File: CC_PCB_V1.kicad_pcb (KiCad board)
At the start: 2 copper layers, 7 parts, among them J1 Screw_Terminal_01x02, J2 Antenna_Conn_02x04_Odd_Even, J3 USB1130-15-A_REVA, J5 Relay_Conn_01x06, U1 Pico, U2 level_converter_BOB-12009

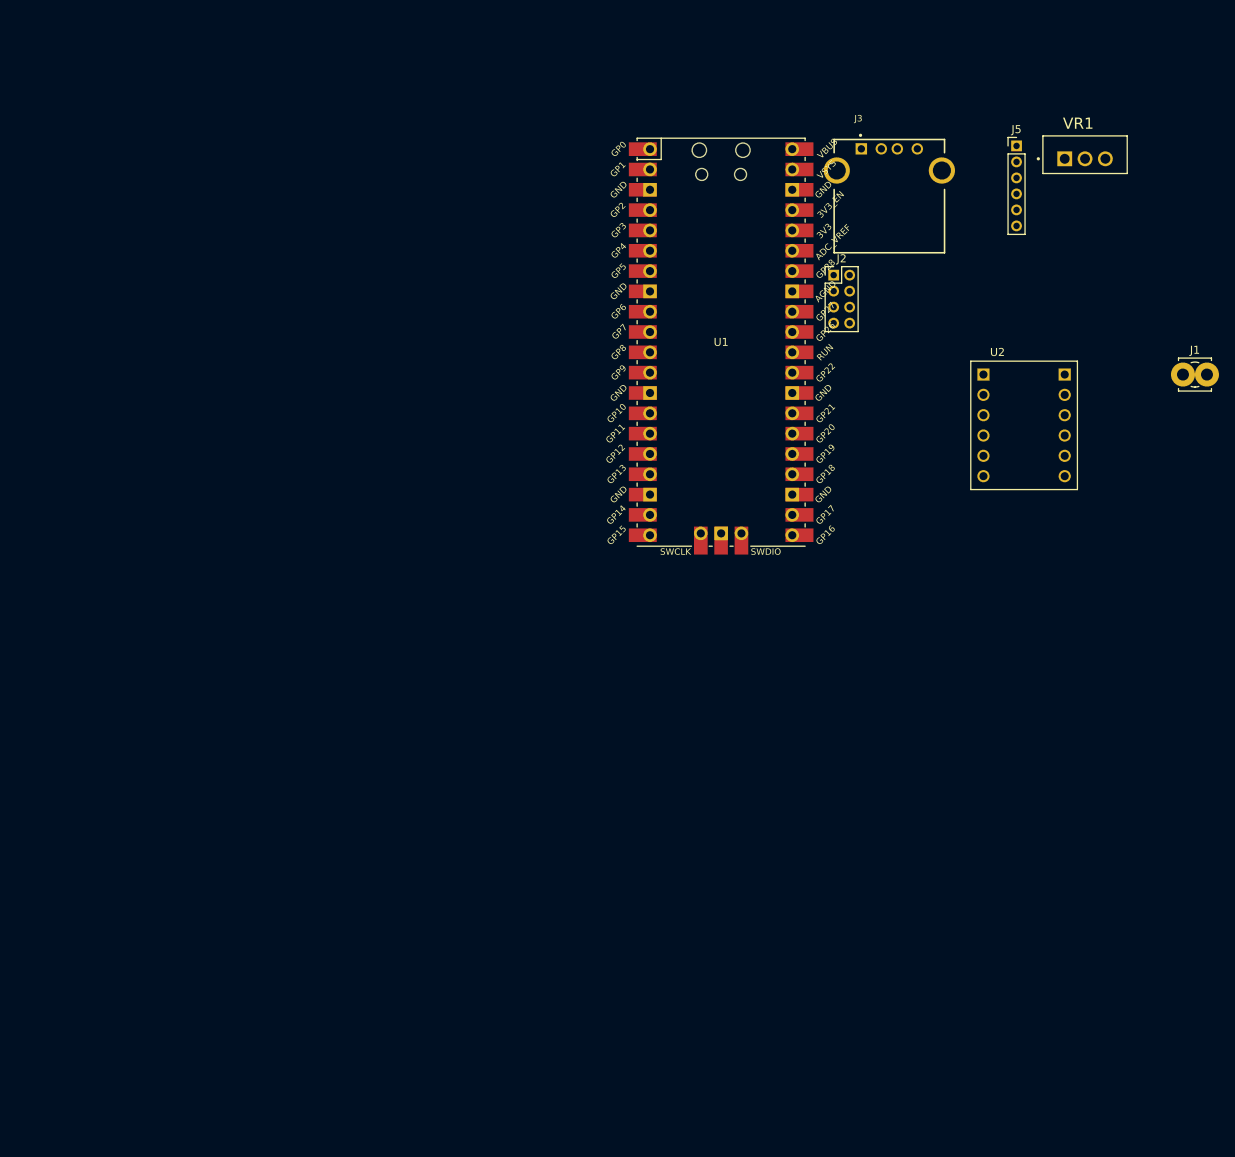
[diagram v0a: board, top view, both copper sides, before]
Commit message: Wiring Board
I tried my best here,  let me know what you think.
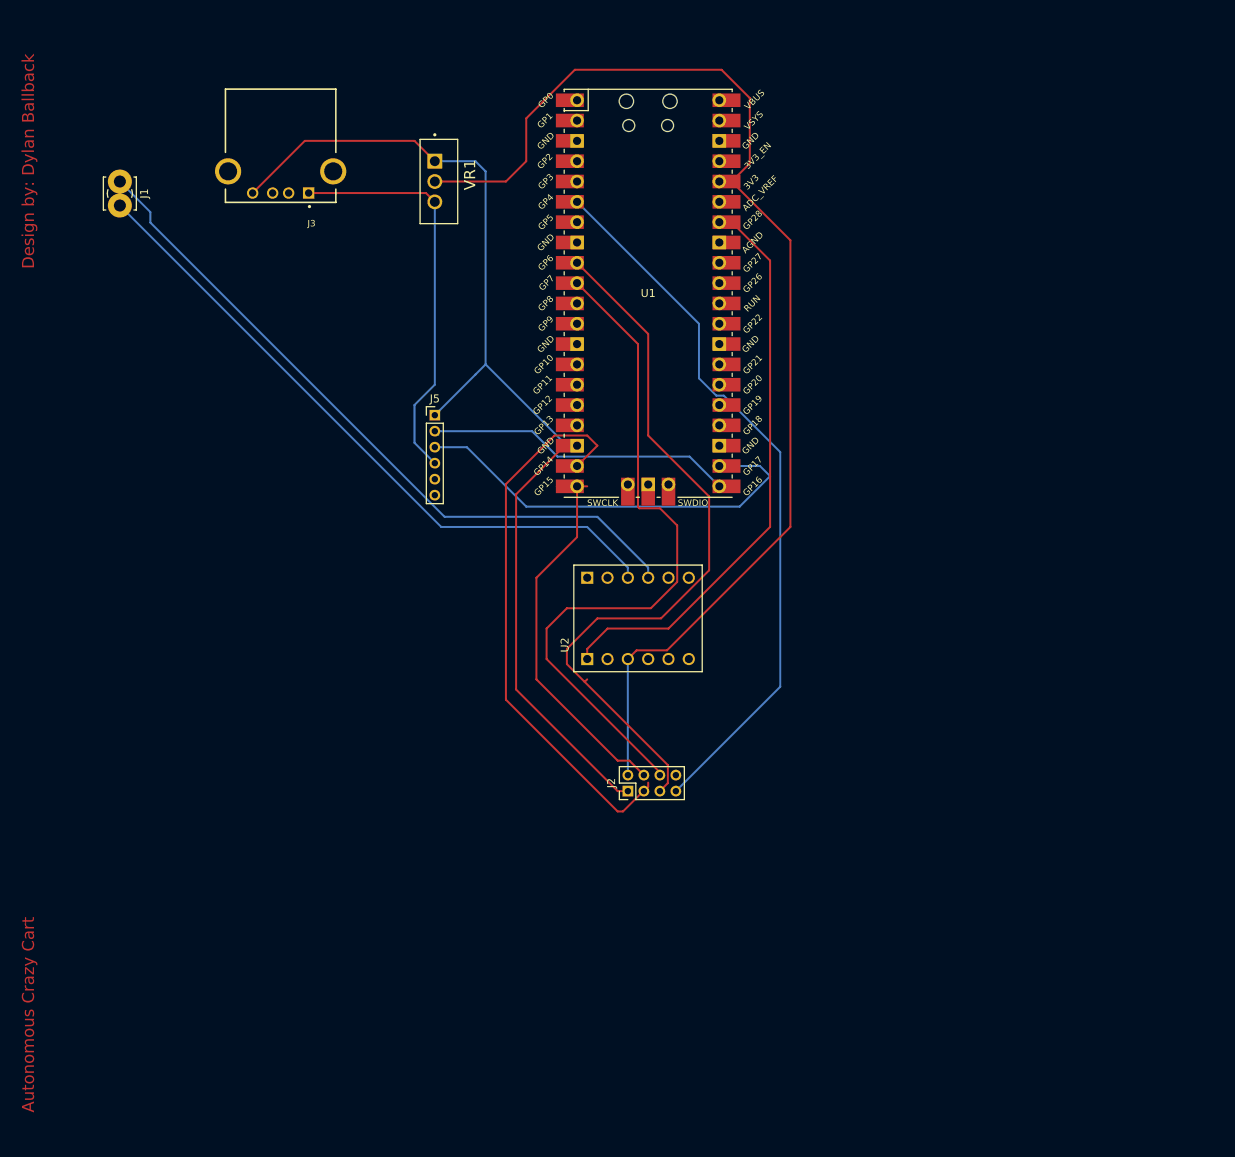
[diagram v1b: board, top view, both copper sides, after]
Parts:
- moved J1 135.1 mm to (71.1, 36.8), turned to 270 degrees
- moved VR1 81.3 mm to (110.5, 36.8), turned to 270 degrees
- moved J5 80.1 mm to (110.5, 66.0)
- moved J3 76.1 mm to (91.2, 35.6), turned to 180 degrees
- moved J2 69.4 mm to (134.6, 113.0), turned to 90 degrees
- moved U2 54.0 mm to (135.9, 91.4), turned to 90 degrees
- moved U1 11.0 mm to (137.2, 50.8)
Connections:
- J1 pad 1: Net-(J1-Pad1) -> GND
- U2 pad GND_1: Net-(J1-Pad2) -> GND
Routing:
- net GND: track 0.00 -> 224.0 mm
- net +3V3: track 0.00 -> 150.6 mm
- net GP6: track 0.00 -> 91.0 mm
- net GP4: track 0.00 -> 90.1 mm
- net GP7: track 0.00 -> 87.0 mm
- net Net-(J1-Pad1): track 0.00 -> 83.5 mm
- net GP28: track 0.00 -> 72.1 mm
- net GP14: track 0.00 -> 70.4 mm
- net GP17: track 0.00 -> 53.4 mm
- net +5V: track 0.00 -> 51.0 mm
- net GP15: track 0.00 -> 48.4 mm
- net GP16: track 0.00 -> 39.0 mm
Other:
- board text added: "Autonomous Crazy Cart"
- board text added: "Design by: Dylan Ballback"
